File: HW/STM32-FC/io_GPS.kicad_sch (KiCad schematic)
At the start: 8 parts, among them J10 GH 1.25mm 6P, J9 GH 1.25mm 10P

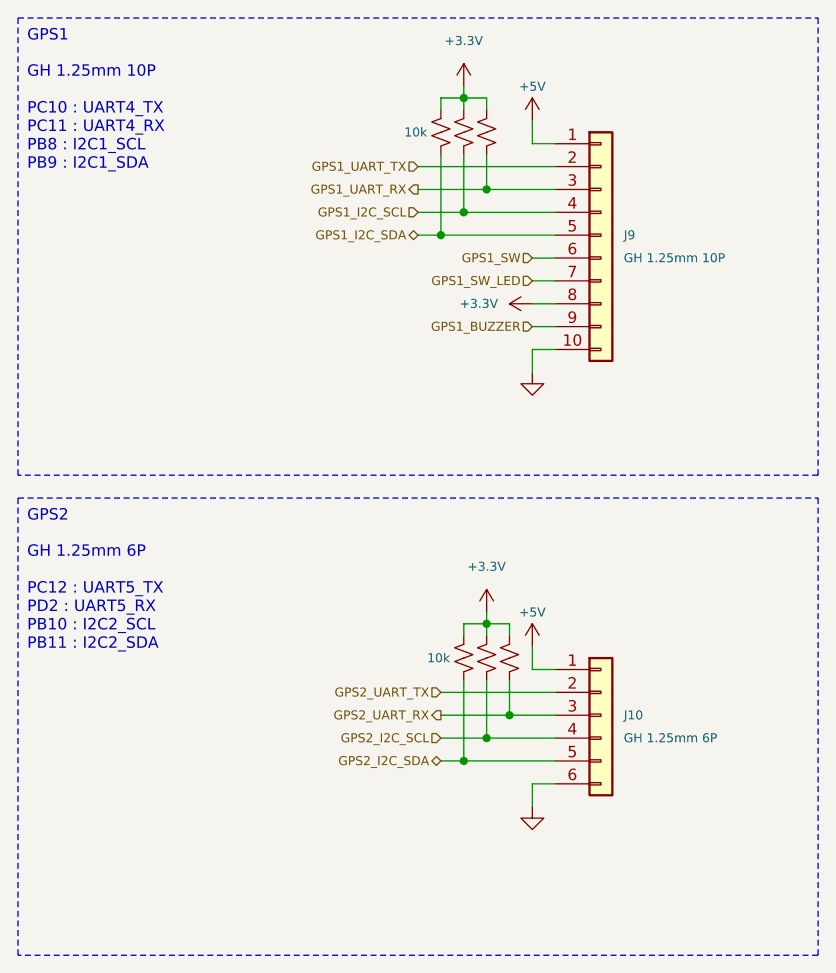
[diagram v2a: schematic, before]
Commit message: 2025.02.06 PCB routing done v2
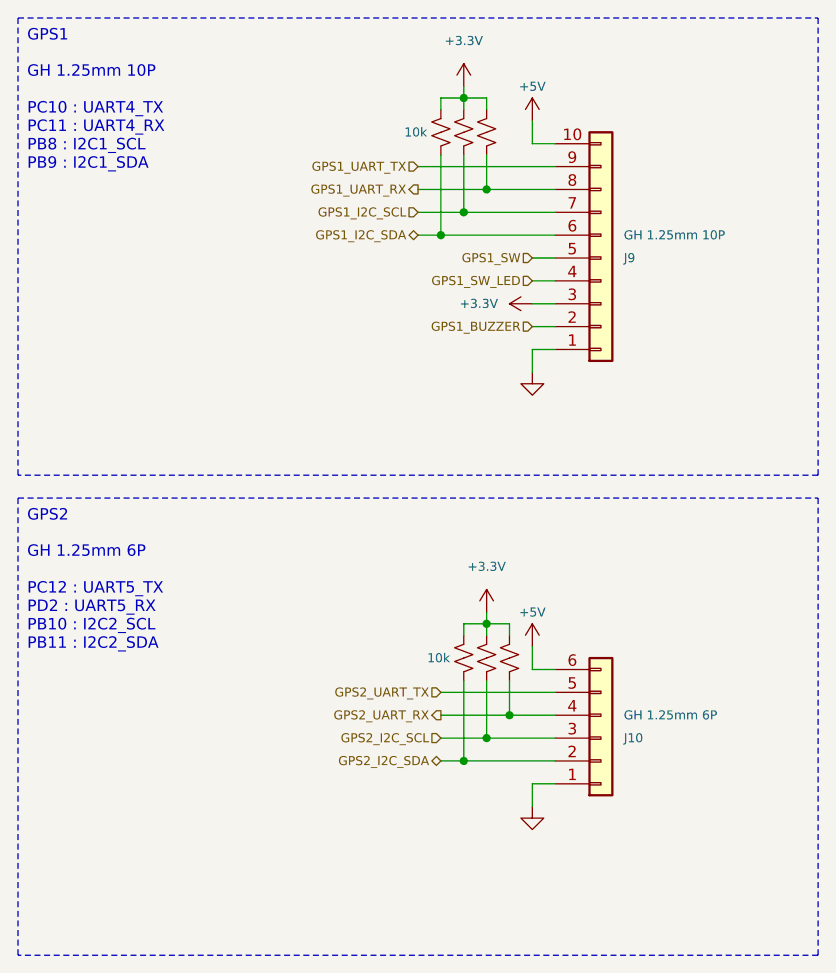
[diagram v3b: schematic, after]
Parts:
- J10: LCSC (none) -> C189892
- J9: LCSC (none) -> C495732
- R23, R24, R25, R26, R27, R28: LCSC (none) -> C25531
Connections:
- net +3.3V: now also J9.3 (Pin_3); no longer J9.8 (Pin_8)
- net +5V: now also J10.6 (Pin_6), J9.10 (Pin_10); no longer J10.1 (Pin_1), J9.1 (Pin_1)
- net GND: now also J10.1 (Pin_1), J9.1 (Pin_1); no longer J10.6 (Pin_6), J9.10 (Pin_10)
- net GPS1_BUZZER: now also J9.2 (Pin_2); no longer J9.9 (Pin_9)
- net GPS1_I2C_SCL: now also J9.7 (Pin_7); no longer J9.4 (Pin_4)
- net GPS1_I2C_SDA: now also J9.6 (Pin_6); no longer J9.5 (Pin_5)
- net GPS1_SW: now also J9.5 (Pin_5); no longer J9.6 (Pin_6)
- net GPS1_SW_LED: now also J9.4 (Pin_4); no longer J9.7 (Pin_7)
- net GPS1_UART_RX: now also J9.8 (Pin_8); no longer J9.3 (Pin_3)
- net GPS1_UART_TX: now also J9.9 (Pin_9); no longer J9.2 (Pin_2)
- net GPS2_I2C_SCL: now also J10.3 (Pin_3); no longer J10.4 (Pin_4)
- net GPS2_I2C_SDA: now also J10.2 (Pin_2); no longer J10.5 (Pin_5)
- net GPS2_UART_RX: now also J10.4 (Pin_4); no longer J10.3 (Pin_3)
- net GPS2_UART_TX: now also J10.5 (Pin_5); no longer J10.2 (Pin_2)
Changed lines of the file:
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@@
+			)
+		)
+		(property "LCSC" "C25531"
+			(at 77.47 83.82 0)
+			(effects
+				(font
+					(size 1.27 1.27)
+				)
+				(hide yes)
 			)
 		)
@@
 			)
 		)
+		(property "LCSC" "C25531"
+			(at 69.85 25.4 0)
+			(effects
+				(font
+					(size 1.27 1.27)
+				)
+				(hide yes)
+			)
+		)
 		(pin "1"
 		)
@@
 	(symbol
 		(lib_id "Connector_Generic:Conn_01x10")
-		(at 87.63 36.83 0)
+		(at 87.63 39.37 0)
+		(mirror x)
 		(unit 1)
 		(exclude_from_sim no)
@@
 		(on_board yes)
 		(dnp no)
-		(fields_autoplaced yes)
 		(property "Reference" "J9"
+			(at 90.17 39.37 0)
+			(effects
+				(font
+					(size 1 1)
+				)
+				(justify left)
+			)
+		)
+		(property "Value" "GH 1.25mm 10P"
 			(at 90.17 36.83 0)
 			(effects
@@
 			)
 		)
-		(property "Value" "GH 1.25mm 10P"
-			(at 90.17 39.37 0)
-			(effects
-				(font
-					(size 1 1)
-				)
-				(justify left)
-			)
-		)
 		(property "Footprint" "JST_GH:JST_GH_BM10B-GHS-TBT_10"
-			(at 87.63 36.83 0)
+			(at 87.63 39.37 0)
 			(effects
 				(font
@@
 		)
 		(property "Datasheet" "~"
-			(at 87.63 36.83 0)
+			(at 87.63 39.37 0)
 			(effects
 				(font
@@
 		)
 		(property "Description" "Generic connector, single row, 01x10, script generated (kicad-library-utils/schlib/autogen/connector/)"
-			(at 87.63 36.83 0)
+			(at 87.63 39.37 0)
 			(effects
 				(font
@@
 		)
 		(property "Availability" ""
-			(at 87.63 36.83 0)
+			(at 87.63 39.37 0)
 			(effects
 				(font
@@
 		)
 		(property "Check_prices" ""
-			(at 87.63 36.83 0)
+			(at 87.63 39.37 0)
 			(effects
 				(font
@@
 		)
 		(property "Description_1" ""
-			(at 87.63 36.83 0)
+			(at 87.63 39.37 0)
 			(effects
 				(font
@@
 		)
 		(property "MF" ""
-			(at 87.63 36.83 0)
+			(at 87.63 39.37 0)
 			(effects
 				(font
@@
 		)
 		(property "MP" ""
-			(at 87.63 36.83 0)
+			(at 87.63 39.37 0)
 			(effects
 				(font
@@
 		)
 		(property "Package" ""
-			(at 87.63 36.83 0)
+			(at 87.63 39.37 0)
 			(effects
 				(font
@@
 		)
 		(property "Price" ""
-			(at 87.63 36.83 0)
+			(at 87.63 39.37 0)
 			(effects
 				(font
@@
 		)
 		(property "SnapEDA_Link" ""
-			(at 87.63 36.83 0)
+			(at 87.63 39.37 0)
 			(effects
 				(font
@@
 		)
 		(property "Sim.Device" ""
-			(at 87.63 36.83 0)
+			(at 87.63 39.37 0)
 			(effects
 				(font
@@
 		)
 		(property "Sim.Pins" ""
-			(at 87.63 36.83 0)
+			(at 87.63 39.37 0)
+			(effects
+				(font
+					(size 1.27 1.27)
+				)
+				(hide yes)
+			)
+		)
+		(property "LCSC" "C495732"
+			(at 87.63 39.37 0)
 			(effects
 				(font
@@
 			)
 		)
+		(property "LCSC" "C25531"
+			(at 72.39 25.4 0)
+			(effects
+				(font
+					(size 1.27 1.27)
+				)
+				(hide yes)
+			)
+		)
 		(pin "1"
 		)
@@
 	(symbol
 		(lib_id "Connector_Generic:Conn_01x06")
-		(at 87.63 90.17 0)
+		(at 87.63 92.71 0)
+		(mirror x)
 		(unit 1)
 		(exclude_from_sim no)
@@
 		(on_board yes)
 		(dnp no)
-		(fields_autoplaced yes)
 		(property "Reference" "J10"
+			(at 90.17 92.71 0)
+			(effects
+				(font
+					(size 1 1)
+				)
+				(justify left)
+			)
+		)
+		(property "Value" "GH 1.25mm 6P"
 			(at 90.17 90.17 0)
 			(effects
@@
 			)
 		)
-		(property "Value" "GH 1.25mm 6P"
-			(at 90.17 92.71 0)
-			(effects
-				(font
-					(size 1 1)
-				)
-				(justify left)
-			)
-		)
 		(property "Footprint" "JST_GH:JST_GH_BM06B-GHS-TBT_06"
-			(at 87.63 90.17 0)
+			(at 87.63 92.71 0)
 			(effects
 				(font
@@
 		)
 		(property "Datasheet" "~"
-			(at 87.63 90.17 0)
+			(at 87.63 92.71 0)
 			(effects
 				(font
@@
 		)
 		(property "Description" "Generic connector, single row, 01x06, script generated (kicad-library-utils/schlib/autogen/connector/)"
-			(at 87.63 90.17 0)
+			(at 87.63 92.71 0)
 			(effects
 				(font
@@
 		)
 		(property "Availability" ""
-			(at 87.63 90.17 0)
+			(at 87.63 92.71 0)
 			(effects
 				(font
@@
 		)
 		(property "Check_prices" ""
-			(at 87.63 90.17 0)
+			(at 87.63 92.71 0)
 			(effects
 				(font
@@
 		)
 		(property "Description_1" ""
-			(at 87.63 90.17 0)
+			(at 87.63 92.71 0)
 			(effects
 				(font
@@
 		)
 		(property "MF" ""
-			(at 87.63 90.17 0)
+			(at 87.63 92.71 0)
 			(effects
 				(font
@@
 		)
 		(property "MP" ""
-			(at 87.63 90.17 0)
+			(at 87.63 92.71 0)
 			(effects
 				(font
@@
 		)
 		(property "Package" ""
-			(at 87.63 90.17 0)
+			(at 87.63 92.71 0)
 			(effects
 				(font
@@
 		)
 		(property "Price" ""
-			(at 87.63 90.17 0)
+			(at 87.63 92.71 0)
 			(effects
 				(font
@@
 		)
 		(property "SnapEDA_Link" ""
-			(at 87.63 90.17 0)
+			(at 87.63 92.71 0)
 			(effects
 				(font
@@
 		)
 		(property "Sim.Device" ""
-			(at 87.63 90.17 0)
+			(at 87.63 92.71 0)
 			(effects
 				(font
@@
 		)
 		(property "Sim.Pins" ""
-			(at 87.63 90.17 0)
+			(at 87.63 92.71 0)
+			(effects
+				(font
+					(size 1.27 1.27)
+				)
+				(hide yes)
+			)
+		)
+		(property "LCSC" "C189892"
+			(at 87.63 92.71 0)
 			(effects
 				(font
@@
 			)
 		)
+		(property "LCSC" "C25531"
+			(at 74.93 25.4 0)
+			(effects
+				(font
+					(size 1.27 1.27)
+				)
+				(hide yes)
+			)
+		)
 		(pin "1"
 		)
@@
 			)
 		)
+		(property "LCSC" "C25531"
+			(at 74.93 83.82 0)
+			(effects
+				(font
+					(size 1.27 1.27)
+				)
+				(hide yes)
+			)
+		)
 		(pin "1"
 		)
@@
 			(at 72.39 83.82 0)
 			(effects
+				(font
+					(size 1.27 1.27)
+				)
+				(hide yes)
+			)
+		)
+		(property "LCSC" "C25531"
+			(at 72.39 83.82 0)
+			(effects

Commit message: 2025.02.06 PCB routing done v3
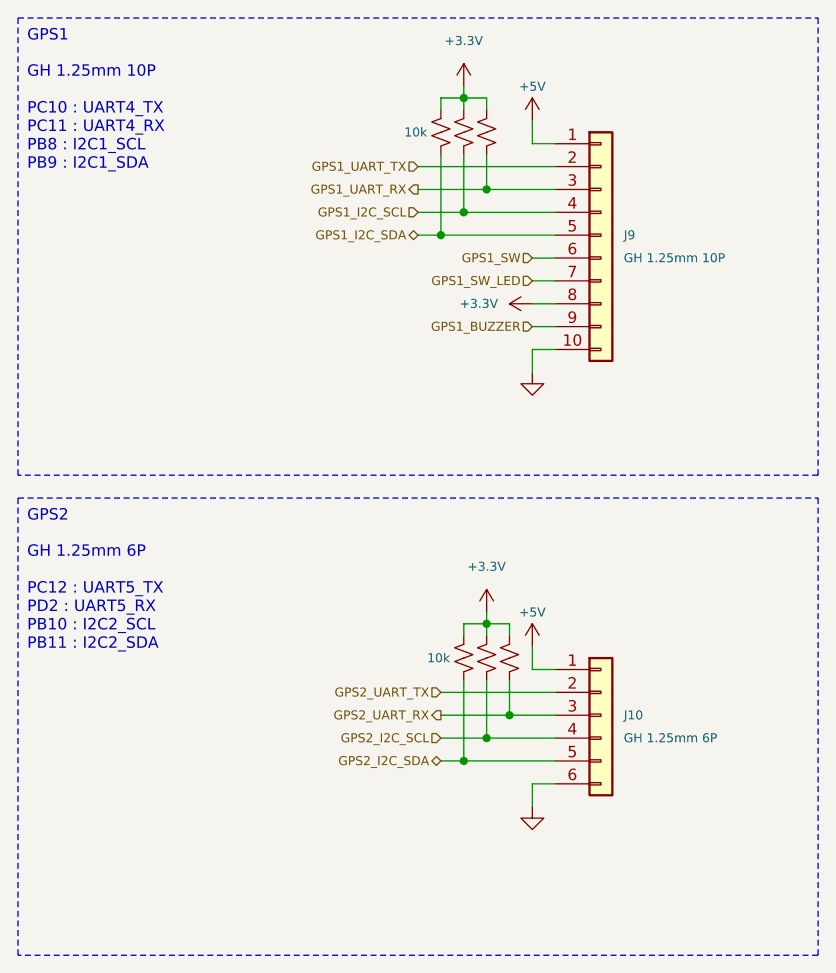
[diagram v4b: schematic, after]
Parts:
- J10: footprint JST_GH:JST_GH_BM06B-GHS-TBT_06 -> JST_GH:JST_GH_SM06B-GHS-TB_06x1.25mm_Angled; LCSC C189892 -> C19626244
- J9: footprint JST_GH:JST_GH_BM10B-GHS-TBT_10 -> JST_GH:JST_GH_SM10B-GHS-TB_10x1.25mm_Angled; LCSC C495732 -> C2683602
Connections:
- net +3.3V: now also J9.8 (Pin_8); no longer J9.3 (Pin_3)
- net +5V: now also J10.1 (Pin_1), J9.1 (Pin_1); no longer J10.6 (Pin_6), J9.10 (Pin_10)
- net GND: now also J10.6 (Pin_6), J9.10 (Pin_10); no longer J10.1 (Pin_1), J9.1 (Pin_1)
- net GPS1_BUZZER: now also J9.9 (Pin_9); no longer J9.2 (Pin_2)
- net GPS1_I2C_SCL: now also J9.4 (Pin_4); no longer J9.7 (Pin_7)
- net GPS1_I2C_SDA: now also J9.5 (Pin_5); no longer J9.6 (Pin_6)
- net GPS1_SW: now also J9.6 (Pin_6); no longer J9.5 (Pin_5)
- net GPS1_SW_LED: now also J9.7 (Pin_7); no longer J9.4 (Pin_4)
- net GPS1_UART_RX: now also J9.3 (Pin_3); no longer J9.8 (Pin_8)
- net GPS1_UART_TX: now also J9.2 (Pin_2); no longer J9.9 (Pin_9)
- net GPS2_I2C_SCL: now also J10.4 (Pin_4); no longer J10.3 (Pin_3)
- net GPS2_I2C_SDA: now also J10.5 (Pin_5); no longer J10.2 (Pin_2)
- net GPS2_UART_RX: now also J10.3 (Pin_3); no longer J10.4 (Pin_4)
- net GPS2_UART_TX: now also J10.2 (Pin_2); no longer J10.5 (Pin_5)
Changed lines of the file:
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@@
+			)
+		)
+		(property "JLC" ""
+			(at 77.47 83.82 0)
+			(effects
+				(font
+					(size 1.27 1.27)
+				)
+				(hide yes)
 			)
 		)
@@
 			)
 		)
+		(property "JLC" ""
+			(at 69.85 25.4 0)
+			(effects
+				(font
+					(size 1.27 1.27)
+				)
+				(hide yes)
+			)
+		)
 		(pin "1"
 		)
@@
 	(symbol
 		(lib_id "Connector_Generic:Conn_01x10")
-		(at 87.63 39.37 0)
-		(mirror x)
+		(at 87.63 36.83 0)
 		(unit 1)
 		(exclude_from_sim no)
@@
 		(dnp no)
 		(property "Reference" "J9"
+			(at 90.17 36.83 0)
+			(effects
+				(font
+					(size 1 1)
+				)
+				(justify left)
+			)
+		)
+		(property "Value" "GH 1.25mm 10P"
 			(at 90.17 39.37 0)
 			(effects
@@
 			)
 		)
-		(property "Value" "GH 1.25mm 10P"
-			(at 90.17 36.83 0)
-			(effects
-				(font
-					(size 1 1)
-				)
-				(justify left)
-			)
-		)
-		(property "Footprint" "JST_GH:JST_GH_BM10B-GHS-TBT_10"
-			(at 87.63 39.37 0)
+		(property "Footprint" "JST_GH:JST_GH_SM10B-GHS-TB_10x1.25mm_Angled"
+			(at 87.63 36.83 0)
 			(effects
 				(font
@@
 		)
 		(property "Datasheet" "~"
-			(at 87.63 39.37 0)
+			(at 87.63 36.83 0)
 			(effects
 				(font
@@
 		)
 		(property "Description" "Generic connector, single row, 01x10, script generated (kicad-library-utils/schlib/autogen/connector/)"
-			(at 87.63 39.37 0)
+			(at 87.63 36.83 0)
 			(effects
 				(font
@@
 		)
 		(property "Availability" ""
-			(at 87.63 39.37 0)
+			(at 87.63 36.83 0)
 			(effects
 				(font
@@
 		)
 		(property "Check_prices" ""
-			(at 87.63 39.37 0)
+			(at 87.63 36.83 0)
 			(effects
 				(font
@@
 		)
 		(property "Description_1" ""
-			(at 87.63 39.37 0)
+			(at 87.63 36.83 0)
 			(effects
 				(font
@@
 		)
 		(property "MF" ""
-			(at 87.63 39.37 0)
+			(at 87.63 36.83 0)
 			(effects
 				(font
@@
 		)
 		(property "MP" ""
-			(at 87.63 39.37 0)
+			(at 87.63 36.83 0)
 			(effects
 				(font
@@
 		)
 		(property "Package" ""
-			(at 87.63 39.37 0)
+			(at 87.63 36.83 0)
 			(effects
 				(font
@@
 		)
 		(property "Price" ""
-			(at 87.63 39.37 0)
+			(at 87.63 36.83 0)
 			(effects
 				(font
@@
 		)
 		(property "SnapEDA_Link" ""
-			(at 87.63 39.37 0)
+			(at 87.63 36.83 0)
 			(effects
 				(font
@@
 		)
 		(property "Sim.Device" ""
-			(at 87.63 39.37 0)
+			(at 87.63 36.83 0)
 			(effects
 				(font
@@
 		)
 		(property "Sim.Pins" ""
-			(at 87.63 39.37 0)
-			(effects
-				(font
-					(size 1.27 1.27)
-				)
-				(hide yes)
-			)
-		)
-		(property "LCSC" "C495732"
-			(at 87.63 39.37 0)
+			(at 87.63 36.83 0)
+			(effects
+				(font
+					(size 1.27 1.27)
+				)
+				(hide yes)
+			)
+		)
+		(property "LCSC" "C2683602 "
+			(at 87.63 36.83 0)
+			(effects
+				(font
+					(size 1.27 1.27)
+				)
+				(hide yes)
+			)
+		)
+		(property "JLC" ""
+			(at 87.63 36.83 0)
 			(effects
 				(font
@@
 			)
 		)
+		(property "JLC" ""
+			(at 72.39 25.4 0)
+			(effects
+				(font
+					(size 1.27 1.27)
+				)
+				(hide yes)
+			)
+		)
 		(pin "1"
 		)
@@
 	(symbol
 		(lib_id "Connector_Generic:Conn_01x06")
-		(at 87.63 92.71 0)
-		(mirror x)
+		(at 87.63 90.17 0)
 		(unit 1)
 		(exclude_from_sim no)
@@
 		(dnp no)
 		(property "Reference" "J10"
+			(at 90.17 90.17 0)
+			(effects
+				(font
+					(size 1 1)
+				)
+				(justify left)
+			)
+		)
+		(property "Value" "GH 1.25mm 6P"
 			(at 90.17 92.71 0)
 			(effects
@@
 			)
 		)
-		(property "Value" "GH 1.25mm 6P"
-			(at 90.17 90.17 0)
-			(effects
-				(font
-					(size 1 1)
-				)
-				(justify left)
-			)
-		)
-		(property "Footprint" "JST_GH:JST_GH_BM06B-GHS-TBT_06"
-			(at 87.63 92.71 0)
+		(property "Footprint" "JST_GH:JST_GH_SM06B-GHS-TB_06x1.25mm_Angled"
+			(at 87.63 90.17 0)
 			(effects
 				(font
@@
 		)
 		(property "Datasheet" "~"
-			(at 87.63 92.71 0)
+			(at 87.63 90.17 0)
 			(effects
 				(font
@@
 		)
 		(property "Description" "Generic connector, single row, 01x06, script generated (kicad-library-utils/schlib/autogen/connector/)"
-			(at 87.63 92.71 0)
+			(at 87.63 90.17 0)
 			(effects
 				(font
@@
 		)
 		(property "Availability" ""
-			(at 87.63 92.71 0)
+			(at 87.63 90.17 0)
 			(effects
 				(font
@@
 		)
 		(property "Check_prices" ""
-			(at 87.63 92.71 0)
+			(at 87.63 90.17 0)
 			(effects
 				(font
@@
 		)
 		(property "Description_1" ""
-			(at 87.63 92.71 0)
+			(at 87.63 90.17 0)
 			(effects
 				(font
@@
 		)
 		(property "MF" ""
-			(at 87.63 92.71 0)
+			(at 87.63 90.17 0)
 			(effects
 				(font
@@
 		)
 		(property "MP" ""
-			(at 87.63 92.71 0)
+			(at 87.63 90.17 0)
 			(effects
 				(font
@@
 		)
 		(property "Package" ""
-			(at 87.63 92.71 0)
+			(at 87.63 90.17 0)
 			(effects
 				(font
@@
 		)
 		(property "Price" ""
-			(at 87.63 92.71 0)
+			(at 87.63 90.17 0)
 			(effects
 				(font
@@
 		)
 		(property "SnapEDA_Link" ""
-			(at 87.63 92.71 0)
+			(at 87.63 90.17 0)
 			(effects
 				(font
@@
 		)
 		(property "Sim.Device" ""
-			(at 87.63 92.71 0)
+			(at 87.63 90.17 0)
 			(effects
 				(font
@@
 		)
 		(property "Sim.Pins" ""
-			(at 87.63 92.71 0)
-			(effects
-				(font
-					(size 1.27 1.27)
-				)
-				(hide yes)
-			)
-		)
-		(property "LCSC" "C189892"
-			(at 87.63 92.71 0)
+			(at 87.63 90.17 0)
+			(effects
+				(font
+					(size 1.27 1.27)
+				)
+				(hide yes)
+			)
+		)
+		(property "LCSC" "C19626244 "
+			(at 87.63 90.17 0)
+			(effects
+				(font
+					(size 1.27 1.27)
+				)
+				(hide yes)
+			)
+		)
+		(property "JLC" ""
+			(at 87.63 90.17 0)
 			(effects
 				(font
@@
 			)
 		)
+		(property "JLC" ""
+			(at 74.93 25.4 0)
+			(effects
+				(font
+					(size 1.27 1.27)
+				)
+				(hide yes)
+			)
+		)
 		(pin "1"
 		)
@@
 			)
 		)
+		(property "JLC" ""
+			(at 74.93 83.82 0)
+			(effects
+				(font
+					(size 1.27 1.27)
+				)
+				(hide yes)
+			)
+		)
 		(pin "1"
 		)
@@
 			(at 72.39 83.82 0)
 			(effects
+				(font
+					(size 1.27 1.27)
+				)
+				(hide yes)
+			)
+		)
+		(property "JLC" ""
+			(at 72.39 83.82 0)
+			(effects

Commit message: 2025.02.07 USB C Conn change v1
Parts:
- J10: LCSC C19626244 -> C133065
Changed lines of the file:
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@@
 			)
 		)
-		(property "LCSC" "C19626244 "
+		(property "LCSC" "C133065"
 			(at 87.63 90.17 0)
 			(effects

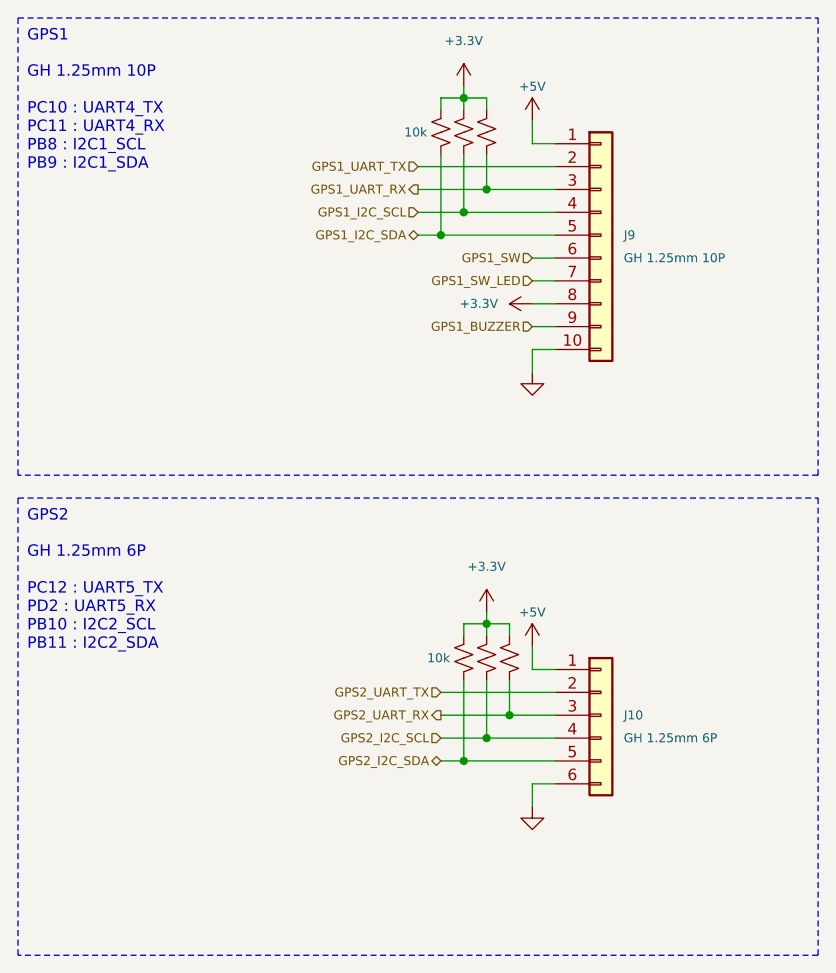
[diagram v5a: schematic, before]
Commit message: 2025.02.11 PCB DONE! MEMO UPDATING
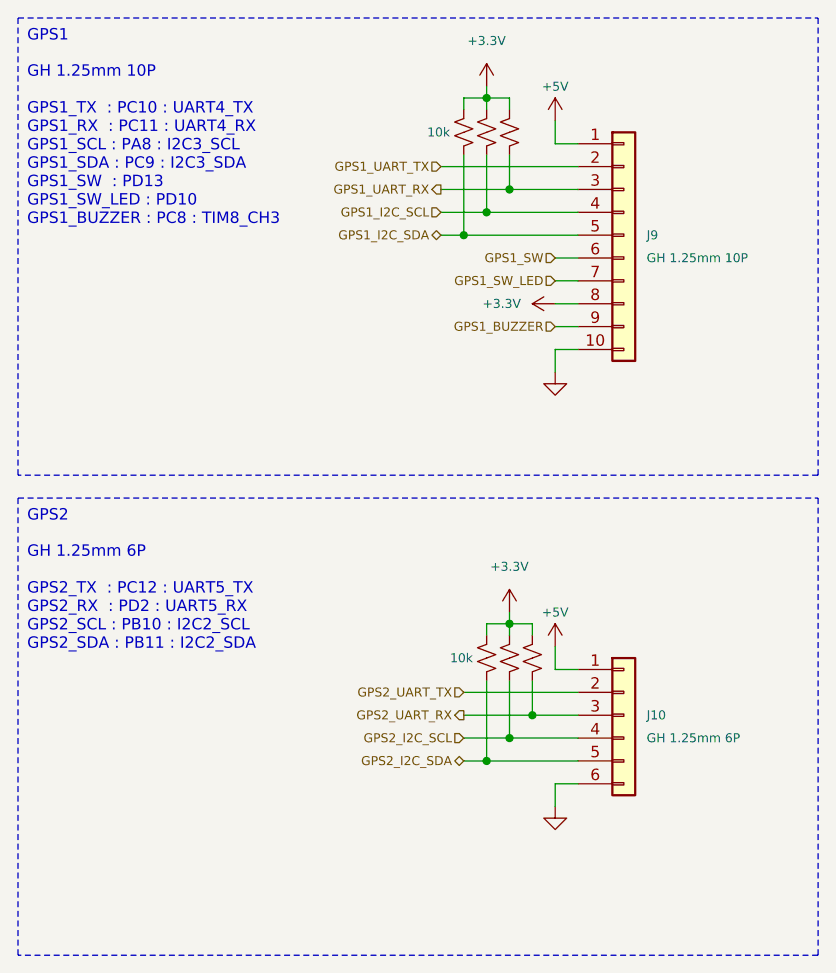
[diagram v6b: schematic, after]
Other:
- note added: "GH 1.25mm 10P GPS1_TX : PC10 : UART4_TX GPS1_RX : PC11 : UART4_RX GPS1_SCL : PA8 : I2C3_SCL GPS1_SDA : PC9 : I2C3_SDA GPS1_SW : PD13 GPS1_SW_LED : PD10 GPS1_BUZZER : PC8 : TIM8_CH3"
- note added: "GH 1.25mm 6P GPS2_TX : PC12 : UART5_TX GPS2_RX : PD2 : UART5_RX GPS2_SCL : PB10 : I2C2_SCL GPS2_SDA : PB11 : I2C2_SDA"
- note removed: "GH 1.25mm 10P PC10 : UART4_TX PC11 : UART4_RX PB8 : I2C1_SCL PB9 : I2C1_SDA"
- note removed: "GH 1.25mm 6P PC12 : UART5_TX PD2 : UART5_RX PB10 : I2C2_SCL PB11 : I2C2_SDA"
- moved on the sheet: J10, J9
